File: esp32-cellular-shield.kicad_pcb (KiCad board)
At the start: 2 copper layers, 68.6 x 53.3 mm, 57 parts, among them Q1 2SC1815, Q2 2SC1815, Q3 2SC1815, Q4 2SC1815, U1 MP2365DN, U2 SIM800, U6 SIM HOLD - PPSS-6P

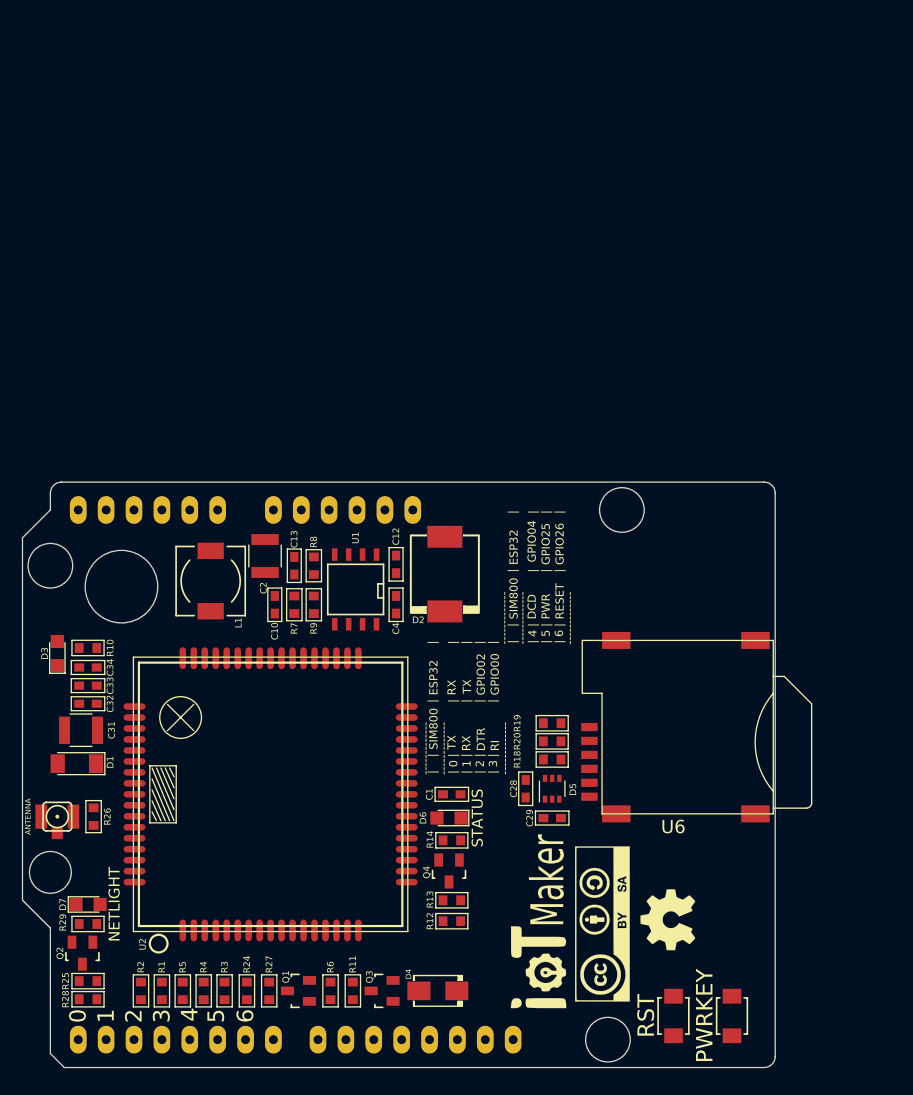
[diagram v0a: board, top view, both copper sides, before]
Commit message: modify esp-uno.lib & add footprint esp-uno-shield
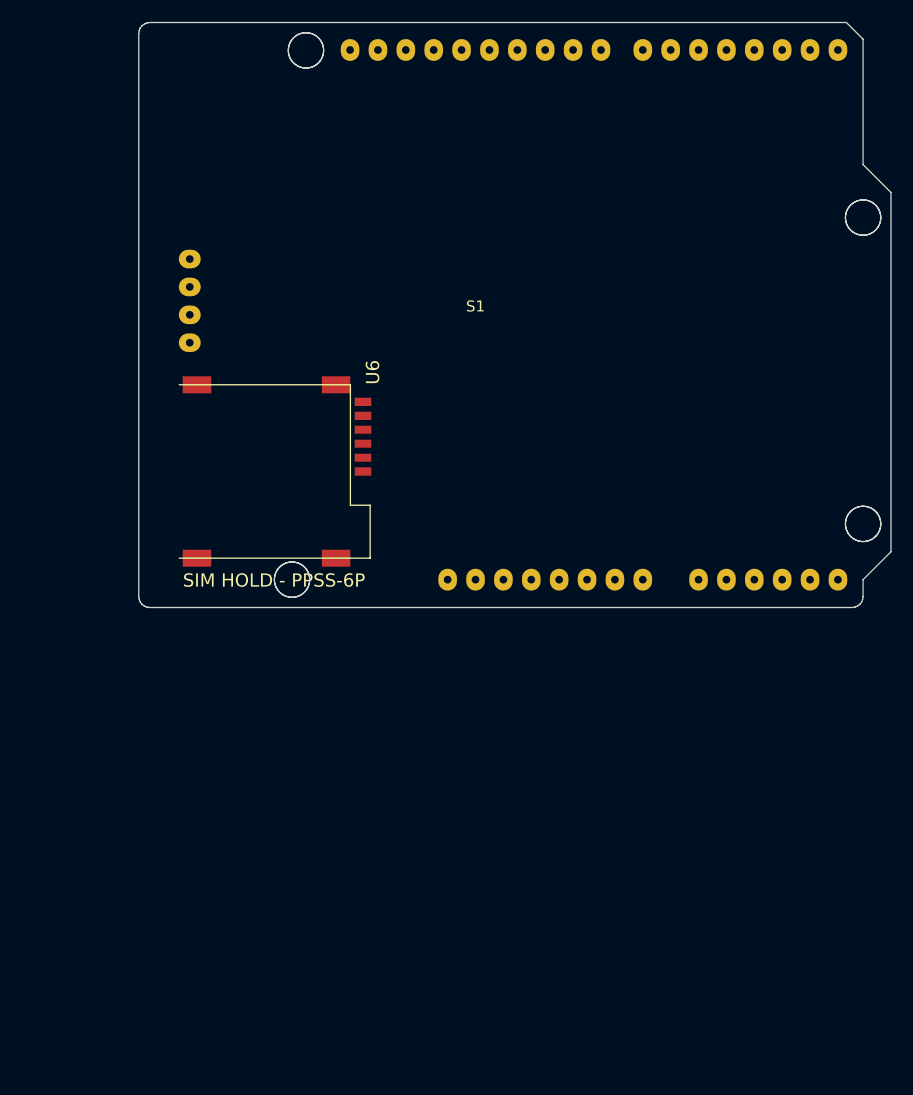
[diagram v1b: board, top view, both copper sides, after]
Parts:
- removed ANT1: ANTENNA, lib:coaxial_u.fl-r-smt-1
- removed C1, C32: 10uF, lib:C_0603
- removed C10: 4.7nF, lib:C_0603
- removed C12: 10nF, lib:C_0603
- removed C13: 47uF, lib:C_0603
- removed C2: 10uF/35V, Capacitors_SMD:C_1210
- removed C28: 100nF, lib:C_0603
- removed C29: 22pF, lib:C_0603
- removed C31: 100uF, Capacitors_SMD:C_1210
- removed C33: 33pF, lib:C_0603
- removed C34: 10pF, lib:C_0603
- removed C4: 0.1uF, lib:C_0603
- removed D1: 5.1V/500mA, Diodes_SMD:D_MiniMELF_Standard
- removed D2: MBRS340, lib:do214ab
- removed D3: Led_pwr, LEDs:LED_0805
- removed D4: D, lib:do214ac
- removed D5: SMF05C, TO_SOT_Packages_SMD:SOT-363_SC-70-6
- removed D6, D7: Led_SIM, LEDs:LED_0805
- removed G***: LOGO, lib:logo_cc-bby-sa_14.1x5mm
- removed G***: LOGO, lib:logo-iotmakervn_7.5x5
- removed L1: 4.7uH-2.2A, Choke_SMD:Choke_SMD_6.3x6.3_H3
- removed PWR1, RST1: SW_PUSH, lib:SW_SPST_B3U-1000P-B
- removed Q1, Q2, Q3, Q4: 2SC1815, lib:SOT-23
- removed R1, R2: 10R, lib:R_0603
- removed R10: 10k, lib:R_0603
- removed R11, R24, R27, R6: 4.7k, lib:R_0603
- removed R12, R13, R25, R28: 4k7, lib:R_0603
- removed R14, R29: 10K, lib:R_0603
- removed R18, R19, R20: 22R, lib:R_0603
- removed R26: 0R, lib:R_0603
- removed R3, R4, R5: 1k, lib:R_0603
- removed R7: 20k, lib:R_0603
- removed R8: 10k-1%, lib:R_0603
- removed R9: 33,6k-1%, lib:R_0603
- removed SHIELD1: ARDUINO_SHIELD, arduino_shields:ARDUINO_SHIELD_2
- removed U1: MP2365DN, SMD_Packages:SOIC-8-N
- removed U2: SIM800, lib:SIM800
- removed VAL**: oshw_logo_500, lib:logo5
- added S1: ESP-UNO, lib:ESP-UNO-SH, F.Cu at (139.7, 76.2)
- moved U6 46.7 mm to (127.0, 83.8), turned to 270 degrees
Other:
- board size 68.6 x 53.3 mm -> 68.5 x 53.3 mm
- board text removed: "-------------"
- board text removed: "0"
- board text removed: "0 1 2 3"
- board text removed: "1"
- board text removed: "2"
- board text removed: "3"
- board text removed: "4"
- board text removed: "4 5 6"
- board text removed: "5"
- board text removed: "6"
- board text removed: "DCD"
- board text removed: "DTR"
- board text removed: "ESP32"
- board text removed: "GPIO00"
- board text removed: "GPIO02"
- board text removed: "GPIO04"
- board text removed: "GPIO25"
- board text removed: "GPIO26"
- board text removed: "Maker"
- board text removed: "NETLIGHT"
- board text removed: "PWR"
- board text removed: "PWRKEY"
- board text removed: "RESET"
- board text removed: "RI"
- board text removed: "RST"
- board text removed: "RX"
- board text removed: "SIM800"
- board text removed: "STATUS"
- board text removed: "TX"
- board text removed: "|"
- board text removed: "| | |"
- board text removed: "| | | |"
